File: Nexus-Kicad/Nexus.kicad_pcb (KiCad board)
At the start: 2 copper layers, 13 parts, among them J1 Conn_01x02_Socket

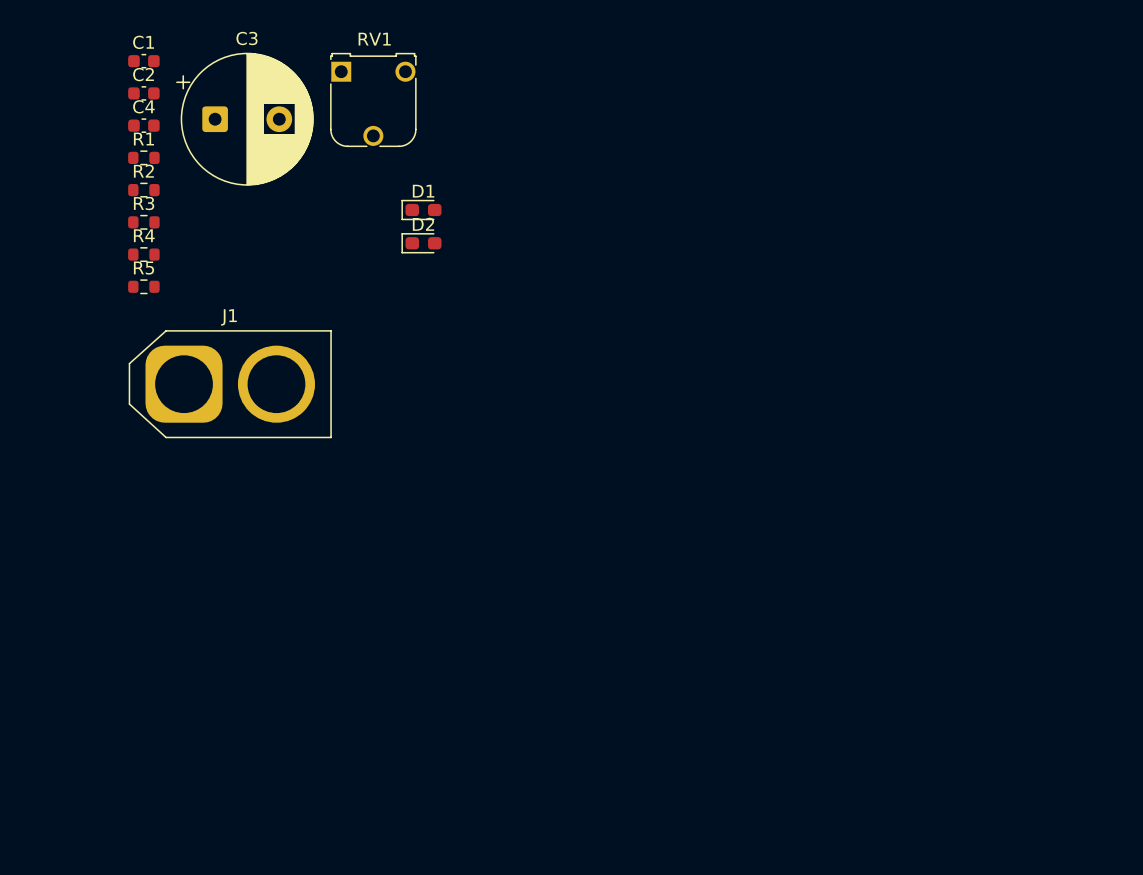
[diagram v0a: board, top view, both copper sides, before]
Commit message: add PCB
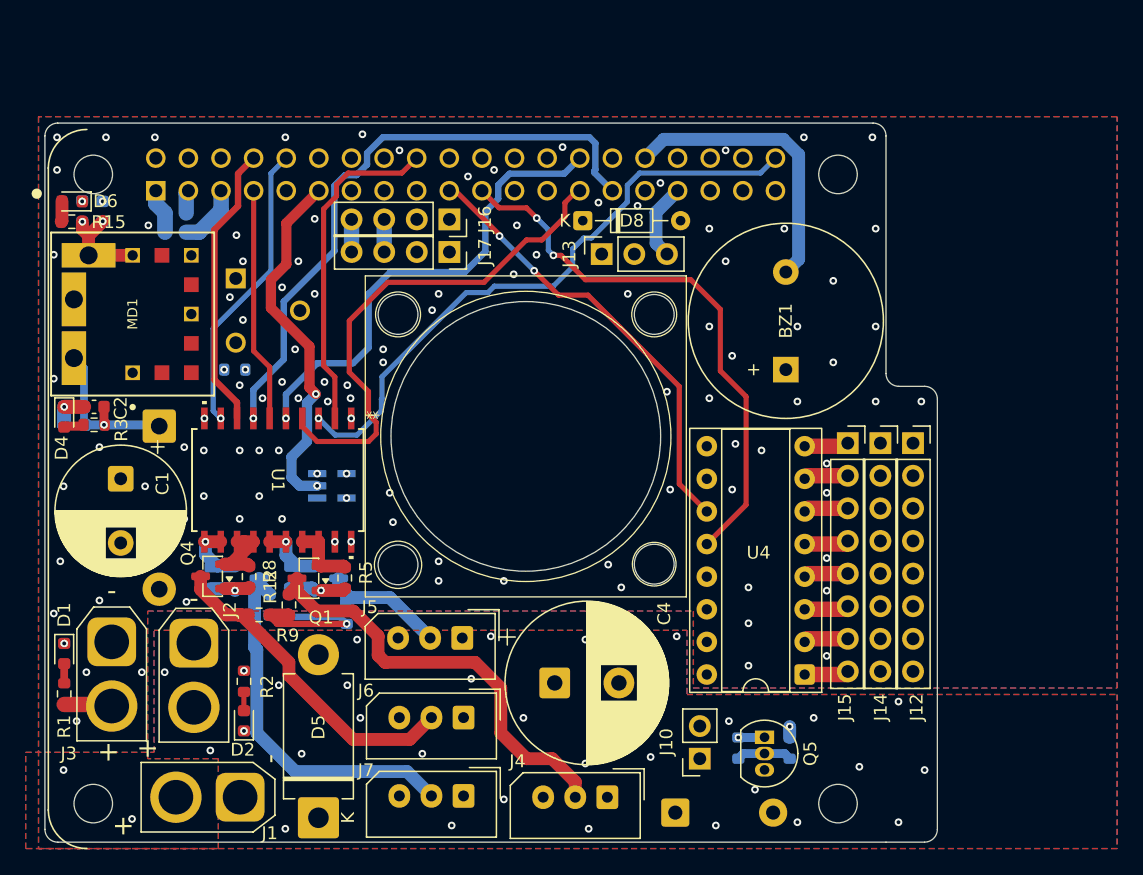
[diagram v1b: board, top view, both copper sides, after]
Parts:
- added BZ1: Buzzer, Buzzer_Beeper:Buzzer_15x7.5RM7.6, F.Cu at (151.9, 79.6)
- added C5: 10uF, Capacitor_SMD:C_0603_1608Metric, B.Cu at (98.7, 67.3)
- added D3: D_Schottky_Filled, Diode_THT:D_DO-201AE_P12.70mm_Horizontal, B.Cu at (103.1, 84.0)
- added D4: LED, LED_SMD:LED_0603_1608Metric, F.Cu at (95.7, 83.3)
- added D5: D_Schottky_Filled, Diode_THT:D_DO-201AD_P12.70mm_Horizontal, F.Cu at (115.5, 114.5)
- added D6: LED, LED_SMD:LED_0603_1608Metric, F.Cu at (96.3, 66.5)
- added D7: 1N4007, Diode_THT:D_DO-41_SOD81_P7.62mm_Horizontal, B.Cu at (143.3, 114.1)
- added D8: D, Diode_THT:D_DO-34_SOD68_P7.62mm_Horizontal, F.Cu at (136.1, 68.0)
- added J10: Conn_01x02_Socket, Connector_PinSocket_2.54mm:PinSocket_1x02_P2.54mm_Vertical, F.Cu at (145.2, 109.9)
- added J12: Conn_01x08_Socket, Connector_PinSocket_2.54mm:PinSocket_1x08_P2.54mm_Vertical, F.Cu at (161.8, 85.3)
- added J13: Conn_01x03_Socket, Connector_PinSocket_2.54mm:PinSocket_1x03_P2.54mm_Vertical, F.Cu at (137.5, 70.6)
- added J14: Conn_01x08_Socket, Connector_PinSocket_2.54mm:PinSocket_1x08_P2.54mm_Vertical, F.Cu at (159.2, 85.3)
- added J15: Conn_01x08_Socket, Connector_PinSocket_2.54mm:PinSocket_1x08_P2.54mm_Vertical, F.Cu at (156.7, 85.3)
- added J16: Conn_01x04_Socket, Connector_PinSocket_2.54mm:PinSocket_1x04_P2.54mm_Vertical, F.Cu at (125.7, 67.9)
- added J17: Conn_01x04_Socket, Connector_PinSocket_2.54mm:PinSocket_1x04_P2.54mm_Vertical, F.Cu at (125.7, 70.5)
- added J2: Conn_01x02_Pin, Connector_AMASS:AMASS_XT30U-F_1x02_P5.0mm_Vertical, F.Cu at (105.8, 100.9)
- added J3: Conn_01x02_Pin, Connector_AMASS:AMASS_XT30U-F_1x02_P5.0mm_Vertical, F.Cu at (99.4, 100.8)
- added J4: Conn_01x03_Socket, Connector_Molex:Molex_SPOX_5267-03A_1x03_P2.50mm_Vertical, F.Cu at (138.0, 112.9)
- added J5: Conn_01x03_Socket, Connector_Molex:Molex_SPOX_5267-03A_1x03_P2.50mm_Vertical, F.Cu at (126.7, 100.5)
- added J6: Conn_01x03_Socket, Connector_Molex:Molex_SPOX_5267-03A_1x03_P2.50mm_Vertical, F.Cu at (126.8, 106.7)
- added J7: Conn_01x03_Socket, Connector_Molex:Molex_SPOX_5267-03A_1x03_P2.50mm_Vertical, F.Cu at (126.8, 112.8)
- added MD1: OKL-T_6-W12N-C, OKLT6W12N:MURATA_OKL-T-6-W12N-C_0, F.Cu at (101.0, 75.3)
- added Q1: BSS138, Package_TO_SOT_SMD:SOT-23, F.Cu at (114.7, 95.9)
- added Q2: BSS138, Package_TO_SOT_SMD:SOT-23, B.Cu at (116.1, 95.9)
- added Q3: BSS138, Package_TO_SOT_SMD:SOT-23, B.Cu at (109.9, 95.9)
- added Q4: BSS138, Package_TO_SOT_SMD:SOT-23, F.Cu at (107.2, 95.7)
- added Q5: 2N7000, Package_TO_SOT_THT:TO-92_Inline, F.Cu at (150.2, 108.2)
- added R10: 2.2k, Resistor_SMD:R_0603_1608Metric, B.Cu at (117.7, 98.6)
- added R11: 2.2k, Resistor_SMD:R_0603_1608Metric, B.Cu at (111.7, 97.9)
- added R12: 2.2k, Resistor_SMD:R_0603_1608Metric, F.Cu at (110.8, 98.7)
- added R13: 1.2k, Resistor_SMD:R_0603_1608Metric, B.Cu at (109.0, 79.6)
- added R14: 1.2k, Resistor_SMD:R_0603_1608Metric, B.Cu at (97.1, 67.3)
- added R15: 1k, Resistor_SMD:R_0603_1608Metric, F.Cu at (96.3, 68.1)
- added R16: 1k, Resistor_SMD:R_0603_1608Metric, B.Cu at (152.2, 109.1)
- added R17: 10k, Resistor_SMD:R_0603_1608Metric, B.Cu at (148.2, 109.1)
- added R18: 1k, Resistor_SMD:R_0603_1608Metric, B.Cu at (104.3, 68.9)
- added R19: 1k, Resistor_SMD:R_0603_1608Metric, B.Cu at (104.3, 67.4)
- added R6: 2.2k, Resistor_SMD:R_0603_1608Metric, B.Cu at (113.3, 95.8)
- added R7: 2.2k, Resistor_SMD:R_0603_1608Metric, B.Cu at (107.1, 95.8)
- added R8: 2.2k, Resistor_SMD:R_0603_1608Metric, F.Cu at (110.1, 95.7)
- added R9: 2.2k, Resistor_SMD:R_0603_1608Metric, F.Cu at (113.2, 97.9)
- added U1: 74HC244D, 74HC244:SOIC20_TOS, F.Cu at (112.3, 88.2)
- added U2: TC7S14F_LF, tc7s14:SOT-25 SMV_TOS, B.Cu at (116.5, 88.7)
- added U3: RASPBERRY_PI_4B_4GB, RaspberryPi4B:MODULE_RASPBERRY_PI_4B_4GB, F.Cu at (136.9, 88.9)
- added U4: MCP3008, Package_DIP:DIP-16_W7.62mm_Socket, F.Cu at (153.3, 103.4)
- C1: value 22uF -> 470uF; footprint Capacitor_SMD:C_0603_1608Metric -> Capacitor_THT:CP_Radial_D10.0mm_P5.00mm
- C2: value 10uF -> 22uF
- C3: value 470uF -> 0.1uF; footprint Capacitor_THT:CP_Radial_D10.0mm_P5.00mm -> Capacitor_SMD:C_0603_1608Metric; moved to B.Cu
- C4: value 0.1uF -> 1000u; footprint Capacitor_SMD:C_0603_1608Metric -> Capacitor_THT:CP_Radial_D12.5mm_P5.00mm
- D1, D2: footprint LED_SMD:LED_0603_1608Metric_Pad1.05x0.95mm_HandSolder -> LED_SMD:LED_0603_1608Metric
- J1: footprint Connector_AMASS:AMASS_XT60-F_1x02_P7.20mm_Vertical -> Connector_AMASS:AMASS_XT30U-F_1x02_P5.0mm_Vertical
- R1: value 20k -> 2k
- R2, R3: value 1.2k -> 2k
- R4: value 2k -> 20k; moved to B.Cu
- R5: value 1k -> 2.2k
- RV1: moved to B.Cu
- moved C4 53.9 mm to (133.9, 104.0)
- moved D1 44.5 mm to (95.7, 101.7), turned to -90 degrees
- moved R1 42.2 mm to (95.7, 104.9), turned to 90 degrees
- moved D2 39.7 mm to (109.7, 107.0), turned to 90 degrees
- moved R2 39.0 mm to (109.7, 103.9), turned to -90 degrees
- moved C1 32.6 mm to (100.1, 88.1), turned to -90 degrees
- moved J1 32.5 mm to (109.4, 112.9), turned to 180 degrees
- moved R5 27.5 mm to (117.5, 95.8), turned to 90 degrees
- moved C3 25.0 mm to (96.4, 82.5), turned to 180 degrees
- moved C2 24.7 mm to (98.0, 82.5), turned to 180 degrees
- moved RV1 18.1 mm to (109.0, 72.5), turned to -90 degrees
- moved R3 16.2 mm to (98.0, 83.9), turned to 180 degrees
- moved R4 14.3 mm to (96.5, 83.9), turned to 180 degrees
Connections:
- C1 pad 2: GNDD -> GNDA
- C2 pad 1: +5V -> Net-(D3-K)
- C2 pad 2: GNDD -> GNDA
- C3 pad 2: GNDD -> GNDA
- C4 pad 1: Net-(D3-K) -> V-Servo
- C4 pad 2: GNDD -> GNDA
- D1 pad 1: GNDD -> GNDA
- D2 pad 1: GNDD -> GNDA
- J1 pad 1: unconnected-(J1-Pin_1-Pad1) -> GNDA
- J1 pad 2: Vcc -> batte
- R1 pad 1: Net-(D3-K) -> batte
- R1 pad 2: GNDD -> Net-(D1-A)
- R2 pad 1: +5V -> +12V
- R2 pad 2: GNDD -> Net-(D2-A)
- R3 pad 1: Net-(R3-Pad1) -> Net-(D3-K)
- R3 pad 2: GNDD -> Net-(D4-A)
- R4 pad 2: Net-(D1-A) -> GNDA
- R5 pad 1: +5V -> 3.3V
- R5 pad 2: Net-(D2-A) -> Servo1_3.3V
- RV1 pad 2: Net-(R3-Pad1) -> Net-(R13-Pad1)
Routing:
- net 3.3V: track 0.00 -> 150.3 mm, vias 0 -> 4
- net RX4: track 0.00 -> 48.2 mm, vias 0 -> 1
- net RX3: track 0.00 -> 47.6 mm, vias 0 -> 1
- net Fan_PWM: track 0.00 -> 45.1 mm, vias 0 -> 1
- net Dout: track 0.00 -> 43.7 mm, vias 0 -> 2
- net Cs: track 0.00 -> 42.2 mm
- net Clock: track 0.00 -> 40.3 mm
- net TX2: track 0.00 -> 39.6 mm
- net RX2: track 0.00 -> 37.3 mm, vias 0 -> 1
- net +5V: track 0.00 -> 35.0 mm, vias 0 -> 51
- net DIn: track 0.00 -> 34.9 mm, vias 0 -> 2
- net Servo1_5V: track 0.00 -> 33.9 mm
- net Enable: track 0.00 -> 33.3 mm, vias 0 -> 3
- net Servo4_5V: track 0.00 -> 29.1 mm
- net Net-(D3-K): track 0.00 -> 26.9 mm, vias 0 -> 1
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- added copper zone on In2.Cu, net +5V
- added copper zone on In4.Cu, net +5V
- added copper zone on B.Cu, net GNDA
- added copper zone on F.Cu, net GNDA
- added copper zone on In1.Cu, net GNDA
- added copper zone on In3.Cu, net GNDA
- added copper zone on In2.Cu, net V-Servo
- added copper zone on In4.Cu, net V-Servo
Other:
- board outline added: 69.5 x 56 mm
- copper layers 2 -> 6
- board text added: "B.T.F-Nexus"
- board text added: "ver 1.0"
